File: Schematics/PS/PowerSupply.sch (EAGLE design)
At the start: 32 parts, among them Q1 BUZ10, Q2 BUZ10

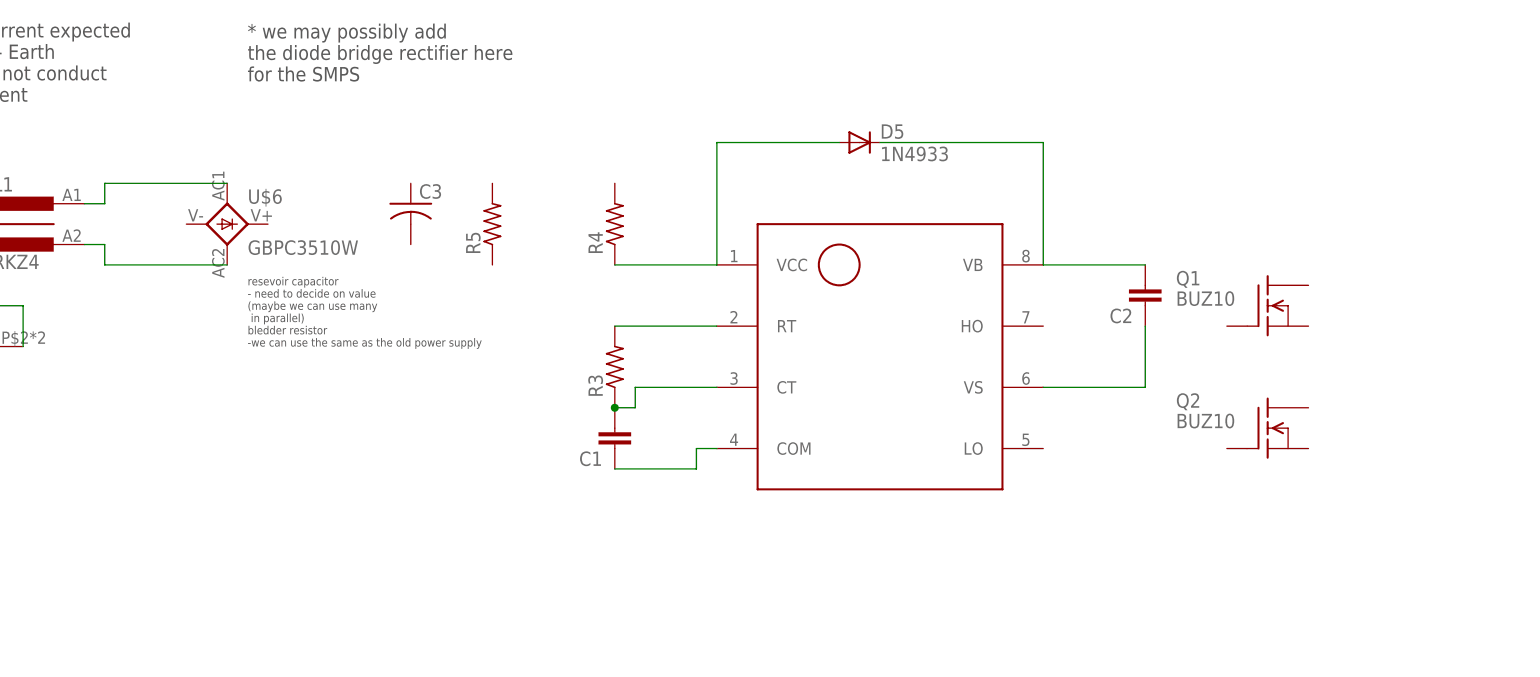
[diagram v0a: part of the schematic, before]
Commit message: updates to PS schematic
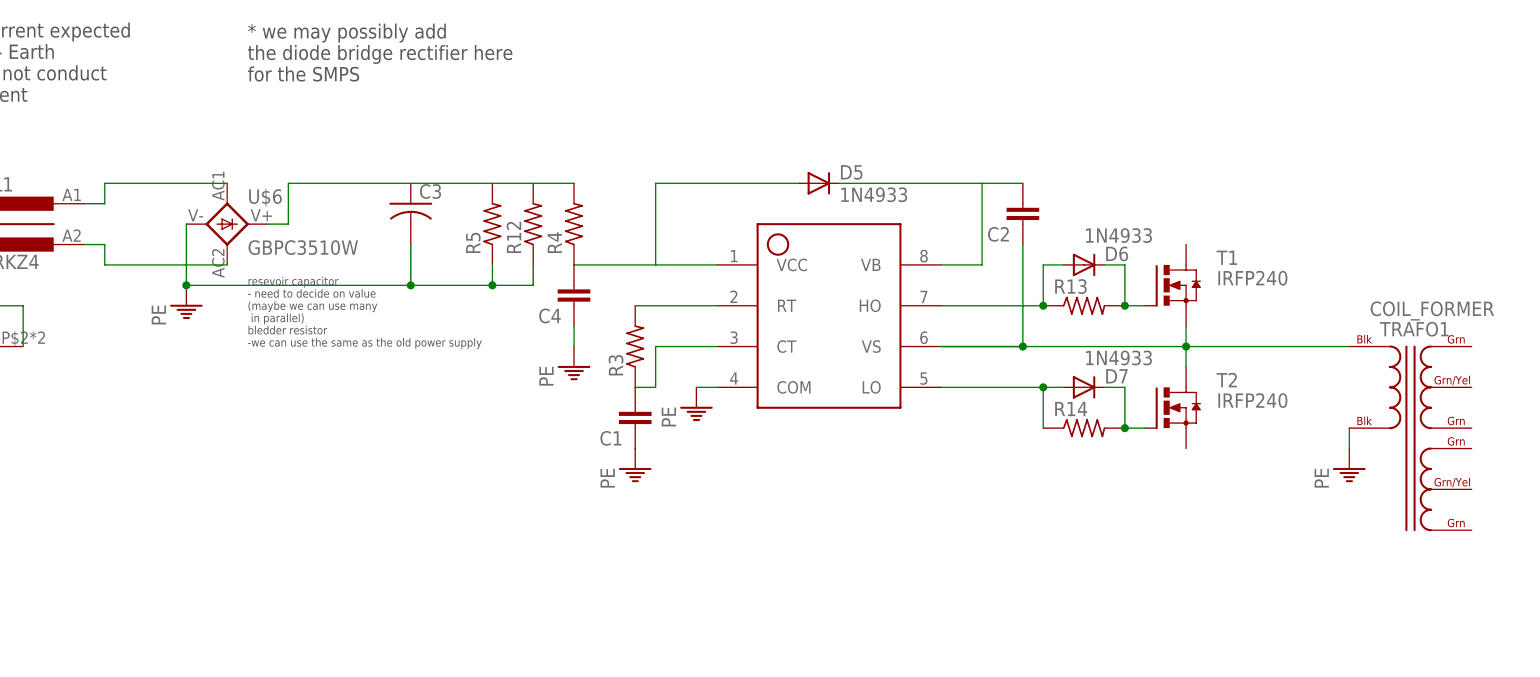
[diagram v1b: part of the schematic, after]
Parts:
- removed Q1, Q2: BUZ10, transistor-fet:BUZ10
- added C4: (no value), resistor:C-EU025-050X050
- added D6, D7: 1N4933, diode:1N4933
- added R12: (no value), resistor:R-US_0617/22
- added R13, R14: (no value), resistor:R-US_0204/2V
- added T1, T2: IRFP240, Amplifier_Parts:IRFP240
- added TRAFO1: COIL_FORMER, Amplifier_Parts:COIL_FORMER
- R5: device resistor:R-US_0309/12 -> resistor:R-US_0617/22
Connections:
- removed net N$13 (its old number): C1.1, U$5.COM
- new net N$19: D6.C, R13.2, T1.G
- new net N$20: D7.A, R14.1, U$5.LO
- new net N$21: D7.C, R14.2, T2.G
- new net N$22: C2.1, T1.S, T2.D, TRAFO1.P1, U$5.VS
- new net N$9: C4.2, D5.A, R4.1, U$5.VCC
- net N$14: now also D6.A, R13.1, U$5.HO; no longer C2.1, U$5.VS
- net N$4: now also C3.1, R12.2, R4.2, R5.2, U$6.+; no longer D5.A, R4.1, U$5.VCC
- net PE: now also C1.1, C3.2, C4.1, R12.1, R5.1, TRAFO1.P15, TRAFO1.P2, U$5.COM, U$6.-
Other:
- moved on the sheet: C1, C2, D5, R3, R4

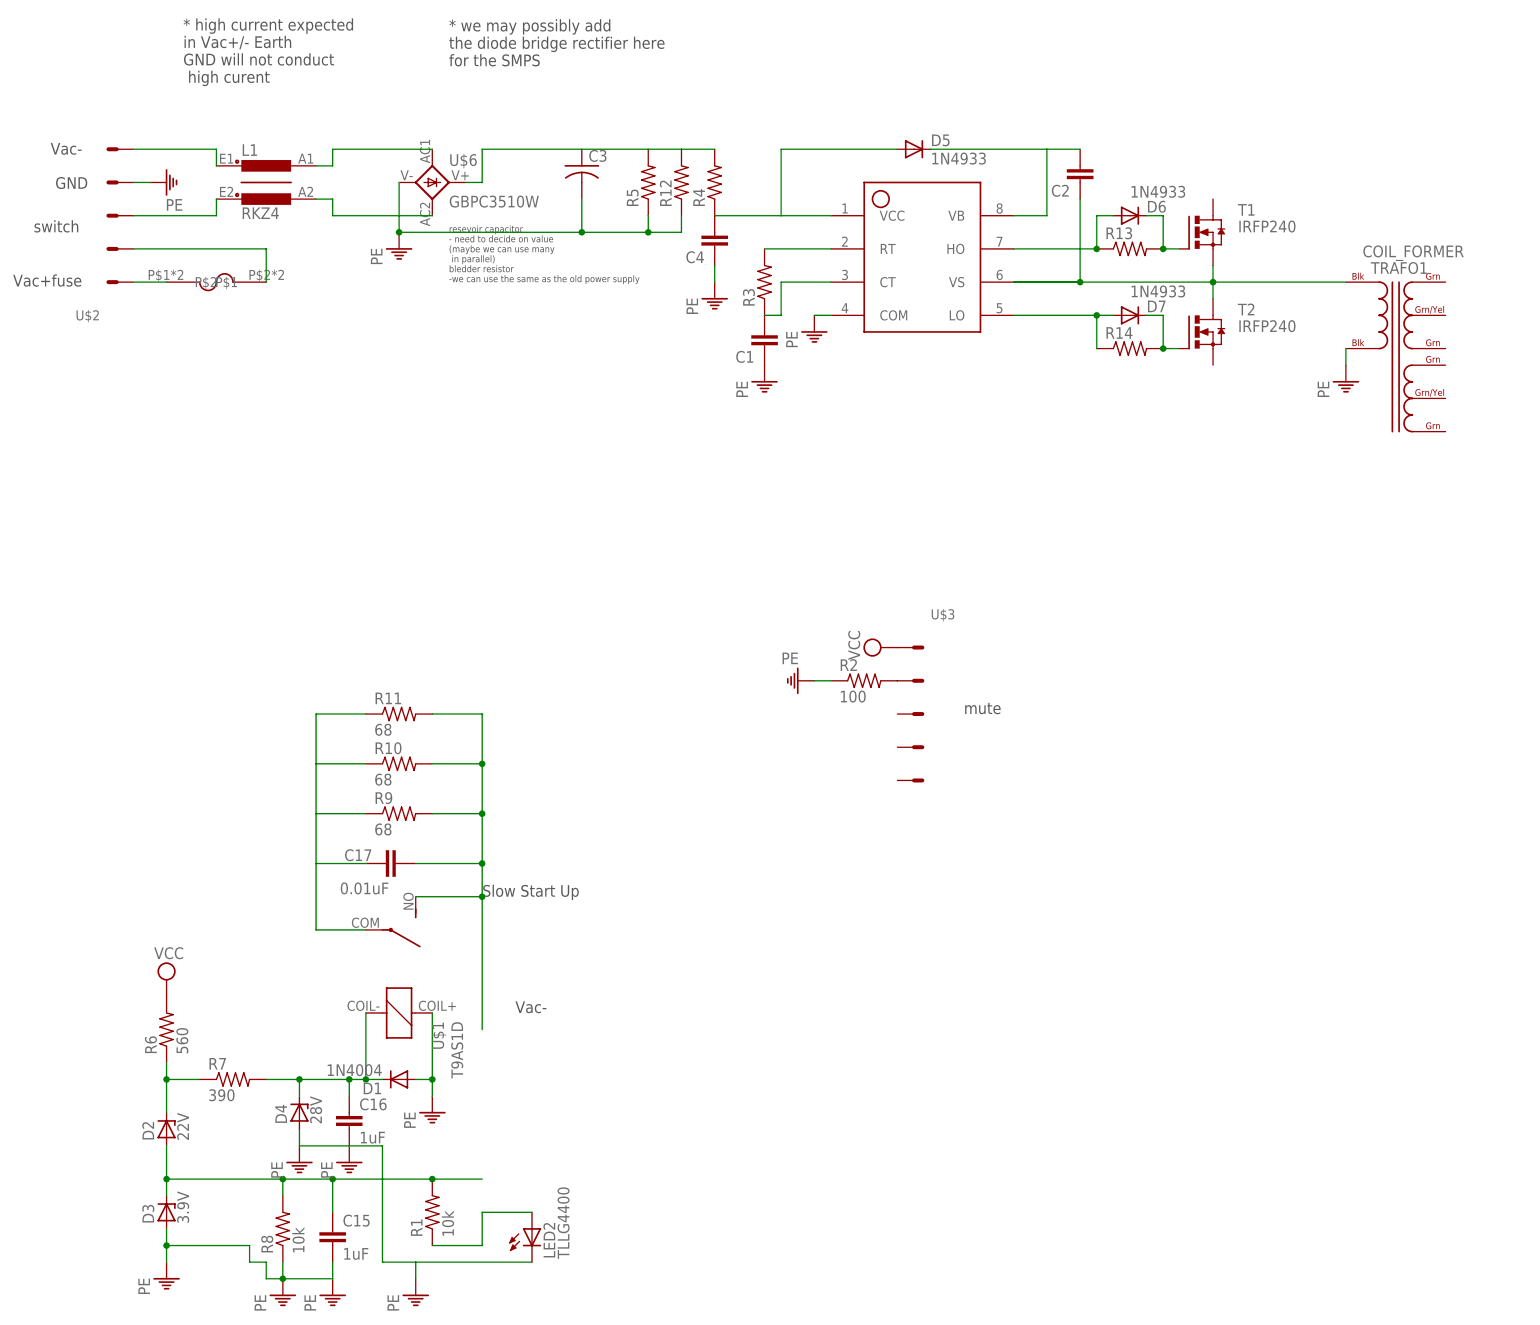
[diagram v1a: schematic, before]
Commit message: updates to PS, libary and Action items
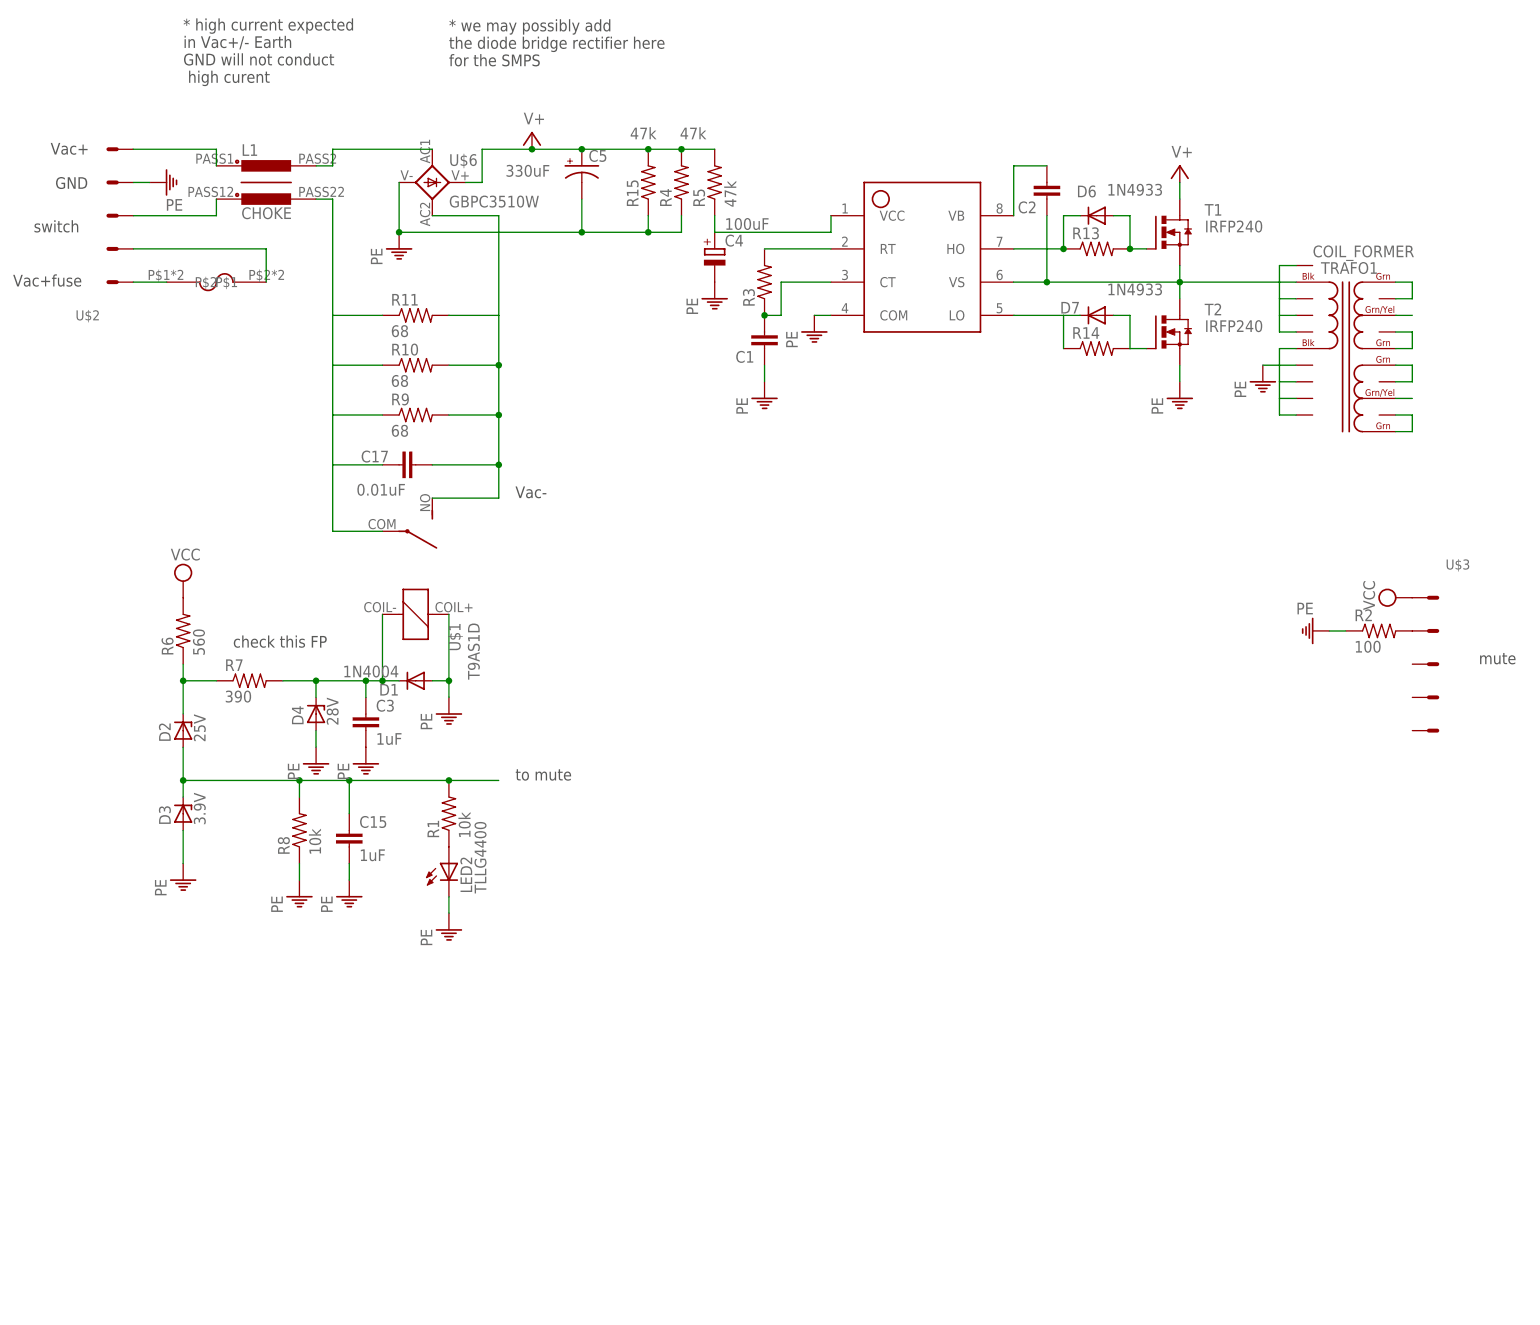
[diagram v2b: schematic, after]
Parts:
- removed C16: 1uF, rcl:C-EU025-060X050
- removed D5: 1N4933, diode:1N4933
- removed R12: (no value), resistor:R-US_0617/22
- added C5: 330uF, rcl:CPOL-USE7.5-18
- added R15: 47k, rcl:R-US_0617/5V
- C1, C2: device resistor:C-EU025-050X050 -> rcl:C-EU050-035X075
- C15: device rcl:C-EU025-060X050 -> rcl:C-EU102-064X133
- C17: device rcl:C-EU025-060X050 -> rcl:C-EU075-042X103
- C3: value (none) -> 1uF; device resistor:C-US050-050X075 -> rcl:C-EU102-064X133
- C4: value (none) -> 100uF; device resistor:C-EU025-050X050 -> rcl:CPOL-EUE2.5-6
- D2: value 22V -> 25V; device diode:ZENER-DIODEP1-12 -> diode:ZENER-DIODEP1-Z12
- D3: device diode:ZENER-DIODEDO34-7 -> diode:ZENER-DIODEZD-2.5
- D4: device diode:ZENER-DIODEP1-12 -> diode:ZENER-DIODEP1-Z12
- L1: value RKZ4 -> CHOKE; device inductors:RKZ4 -> Amplifier_Parts:CHOKE
- R1, R7, R8: device resistor:R-US_0207/15 -> rcl:R-US_0204/2V
- R10, R11, R9: device rcl:R-US_0617/22 -> rcl:R-US_0617/5V
- R3: device resistor:R-US_0309/10 -> rcl:R-US_0204/2V
- R4: value (none) -> 47k; device resistor:R-US_0309/10 -> rcl:R-US_0617/5V
- R5: value (none) -> 47k; device resistor:R-US_0617/22 -> rcl:R-US_0617/5V
- R6: device resistor:R-US_0207/15 -> rcl:R-US_0309/V
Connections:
- removed net N$4 (its old number): C3.1, R12.2, R4.2, R5.2, U$6.+
- removed net N$8: C17.2, R10.2, R11.2, R9.2, U$1.NO
- removed net VAC-: C17.1, R10.1, R11.1, R9.1, U$1.COM
- new net N$17: C4.+, R5.1, U$5.VCC
- new net N$24: TRAFO1.S30+1, TRAFO1.SEC30V+
- new net N$25: TRAFO1.GND30
- new net N$26: TRAFO1.S15+1, TRAFO1.SEC15+
- new net N$27: TRAFO1.S15-1, TRAFO1.SEC15-
- new net N$28: TRAFO1.GND15
- new net V+: C5.+, R15.2, R4.2, R5.2, T1.D, U$6.+
- net GND: now also C1.1, C17.1, C5.-, L1.W2E, R10.1, R11.1, R15.1, R4.1, R9.1, T2.S, TRAFO1.P2, TRAFO1.P22, TRAFO1.P23, TRAFO1.P24, TRAFO1.P25, U$1.COM, U$5.COM, U$6.-; no longer C16.2
- net N$10: now also C3.1; no longer C16.1
- net N$14: now also D6.C; no longer D6.A
- net N$18: now also C17.2, R10.2, R11.2, R9.2, U$1.NO; no longer L1.W2E
- net N$19: now also D6.A; no longer D6.C
- net N$20: now also D7.C; no longer D7.A
- net N$21: now also D7.A; no longer D7.C
- net N$22: now also TRAFO1.P12, TRAFO1.P13, TRAFO1.P14, TRAFO1.P15
- net N$6: no longer D5.C
- net N$9: now also TRAFO1.S30-1, TRAFO1.SEC30-; no longer C4.2, D5.A, R4.1, U$5.VCC
- net PE: no longer C1.1, C4.1, R12.1, R5.1, TRAFO1.P15, TRAFO1.P2, U$5.COM, U$6.-
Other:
- note added: "Vac+"
- note added: "check this FP"
- note added: "to mute"
- note removed: "Slow Start Up"
- note removed: "resevoir capacitor - need to decide on value (maybe we can use many in parallel) bledder resistor -we can use the same as the old power supply"
- moved on the sheet: C15, C17, C2, C3, D1, D2, D3, D4, D6, D7, LED2, R1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
